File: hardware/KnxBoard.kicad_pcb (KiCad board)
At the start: 2 copper layers, 45 parts, among them J1 Conn_01x12_Male, J2 Conn_01x12, J3 Conn_01x12, J4 Conn_01x02_Male, SW1 SW_Push, SW2 SW_Push, U1 NCN5130, U2 STM32L432KCUx, X1 FA-238

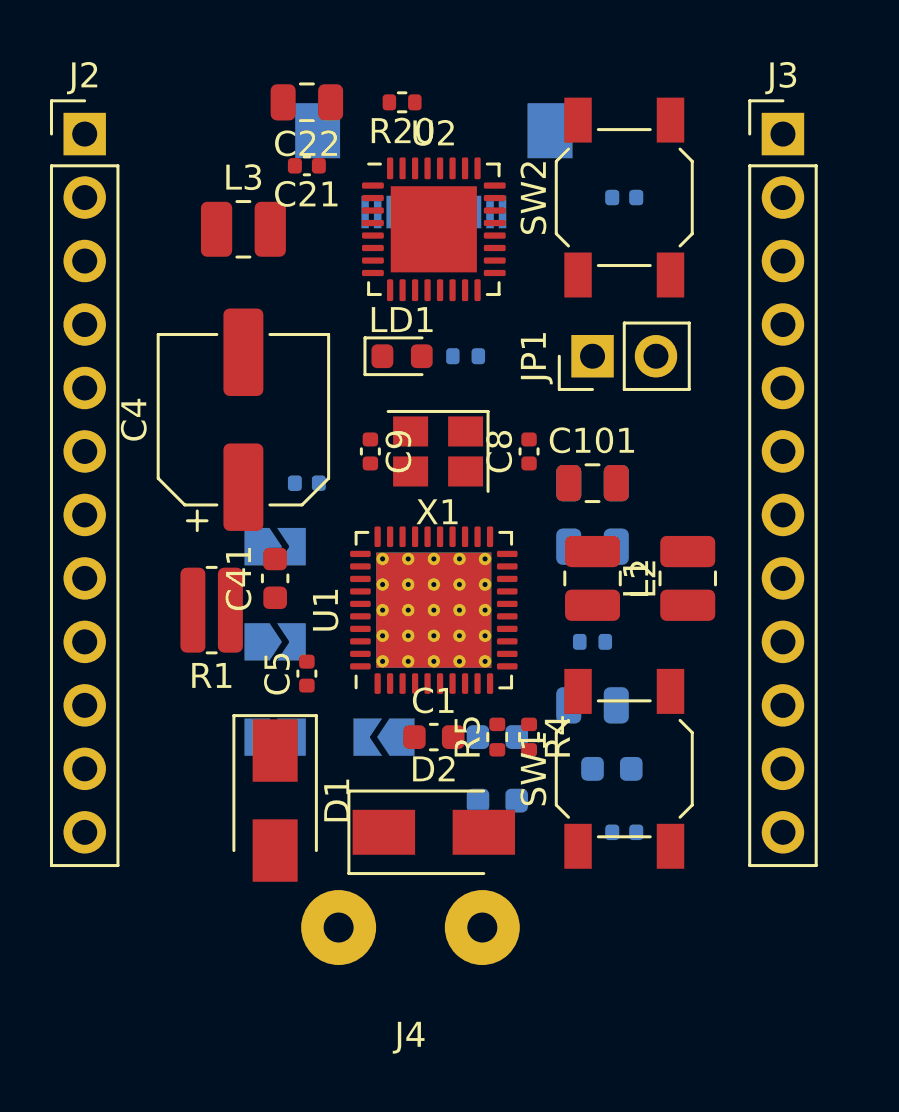
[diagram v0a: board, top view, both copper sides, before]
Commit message: KnxBoard: Continue with layer 2
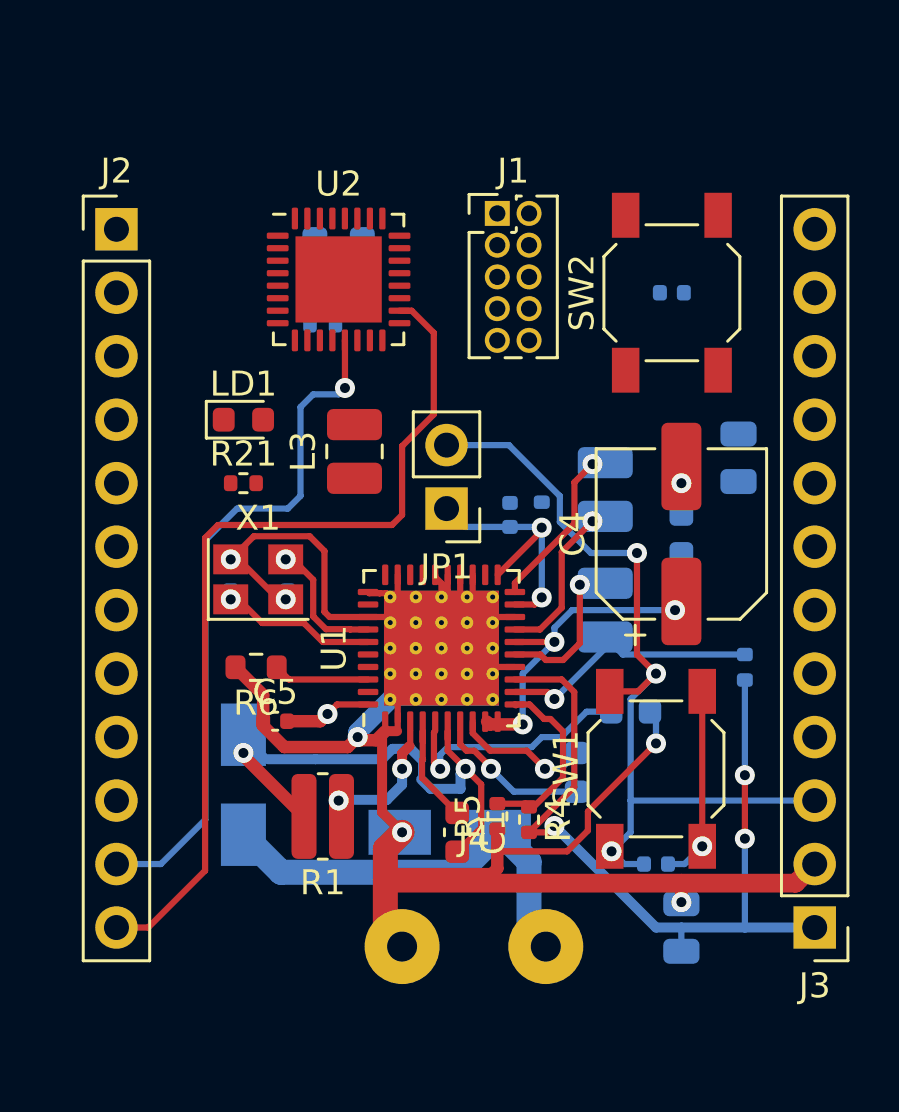
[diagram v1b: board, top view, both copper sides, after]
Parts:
- removed C101, C111: 10uF 6.3V ESR < 0.1ohm, Capacitor_SMD:C_0805_2012Metric
- removed C7: 1uF 35V ESR < 2ohm, Capacitor_SMD:C_0603_1608Metric
- removed JP2, JP3, JP4, JP5: SolderJumper_2_Open, Jumper:SolderJumper-2_P1.3mm_Open_TrianglePad1.0x1.5mm
- added R6: NOTMOUNT, Resistor_SMD:R_0603_1608Metric, F.Cu at (140.2, 111.5)
- C21, C22, C41, C8, C9, D1, D2, L1, L2, R20: moved to B.Cu
- J1: value Conn_01x12_Male -> Conn_01x10; footprint Connector_FFC-FPC:Hirose_FH12-12S-0.5SH_1x12-1MP_P0.50mm_Horizontal -> Connector_PinHeader_1.27mm:PinHeader_2x05_P1.27mm_Vertical; moved to F.Cu
- R21: moved to F.Cu
- moved J3 31.8 mm to (162.6, 121.9), turned to 180 degrees
- moved C4 18.1 mm to (157.2, 106.2)
- moved C41 16.4 mm to (157.2, 106.2)
- moved C11 15.6 mm to (157.2, 121.9), turned to 90 degrees
- moved C8 13.0 mm to (139.2, 108.0), turned to 270 degrees
- moved R21 10.2 mm to (139.7, 104.1), turned to 0 degrees
- moved L3 9.94 mm to (144.1, 102.9), turned to 90 degrees
- moved R20 9.44 mm to (142.9, 97.8)
- moved R1 9.38 mm to (142.9, 117.5)
- moved X1 8.83 mm to (140.3, 108.0), turned to 0 degrees
- moved JP1 8.44 mm to (147.8, 105.2), turned to 180 degrees
- moved C6 8.23 mm to (150.4, 105.4), turned to 90 degrees
- moved J4 7.31 mm to (148.9, 118.9), turned to 180 degrees
- moved LD1 6.84 mm to (139.7, 101.6)
- moved R3 6.18 mm to (159.8, 111.5), turned to 270 degrees
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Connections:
- net Net-(C8-Pad2) renamed /CLK0
- net Net-(C9-Pad2) renamed /CLK1
- C4 pad 1: Net-(C4-Pad1) -> /Vfilt
- C41 pad 1: Net-(C4-Pad1) -> /Vfilt
- J1 pad 1: GND -> Net-(J1-Pad1)
- J1 pad 10: NRST -> VDD
- J1 pad 2: SWCLK -> GND
- J1 pad 3: SWDIO -> NRST
- J1 pad 4: TXD -> UART_RX
- J1 pad 5: RXD -> UART_TX
- J1 pad 6: UART_TX -> SWCLK
- J1 pad 7: UART_RX -> SWDIO
- J1 pad 8: CLK16 -> TXD
- J1 pad 9: RESETB -> RXD
- U1 pad 10: Net-(C7-Pad1) -> /Vfilt
- U1 pad 16: Net-(C4-Pad1) -> /Vfilt
- U1 pad 21: Net-(U1-Pad21) -> +3V3
- U1 pad 36: SAVEB -> PA11
- U1 pad 37: RESETB -> NRST
- U1 pad 41: (no net) -> GND
- U1 pad 9: Net-(C4-Pad1) -> /Vfilt
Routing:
- net GND: track 0.00 -> 99.7 mm, vias 0 -> 7
- net PA8: track 0.00 -> 35.6 mm
- net VDD: track 0.00 -> 34.0 mm, vias 0 -> 3
- net +12V: track 0.00 -> 33.0 mm, vias 0 -> 3
- net PA7: track 0.00 -> 27.6 mm, vias 0 -> 1
- net Net-(C1-Pad2): track 0.00 -> 22.3 mm, vias 0 -> 2
- net /KNX+: track 0.00 -> 15.8 mm
- net /Vfilt: track 0.00 -> 15.1 mm, vias 0 -> 3
- net +3V3: track 0.00 -> 14.2 mm, vias 0 -> 3
- net Net-(L2-Pad2): track 0.00 -> 10.9 mm, vias 0 -> 1
- net Net-(C3-Pad1): track 0.00 -> 9.75 mm, vias 0 -> 1
- net Prog: track 0.00 -> 7.86 mm, vias 0 -> 1
- net Net-(R4-Pad1): track 0.00 -> 7.44 mm
- net /CLK0: track 0.00 -> 6.56 mm, vias 0 -> 1
- net Net-(L1-Pad2): track 0.00 -> 6.40 mm, vias 0 -> 1
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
